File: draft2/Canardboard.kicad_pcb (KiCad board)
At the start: 4 copper layers, 96.5 x 62 mm, 112 parts, among them IC1 SIC437DED-T1-GE3, J1 RBUS, J2 USB_C_Receptacle_USB2.0, J3 Micro_SD_Card_Det, J4 Conn_01x02_Male, J5 Conn_01x03_Male, J6 Conn_01x03_Male, J7 Conn_01x03_Male, Q1 SI4143DY-T1-GE3, Q2 SI4143DY-T1-GE3, U1 ESP32-S3, U10 LTC4412xS6, U2 SN65HVD230, U3 LM66200DRLR, U5 MAX77827AEFD+T, U6 SC4215, U7 ICM-20608-G, U8 MMC5983MA, U9 LTC4412xS6, Y1 40MHz±10ppm

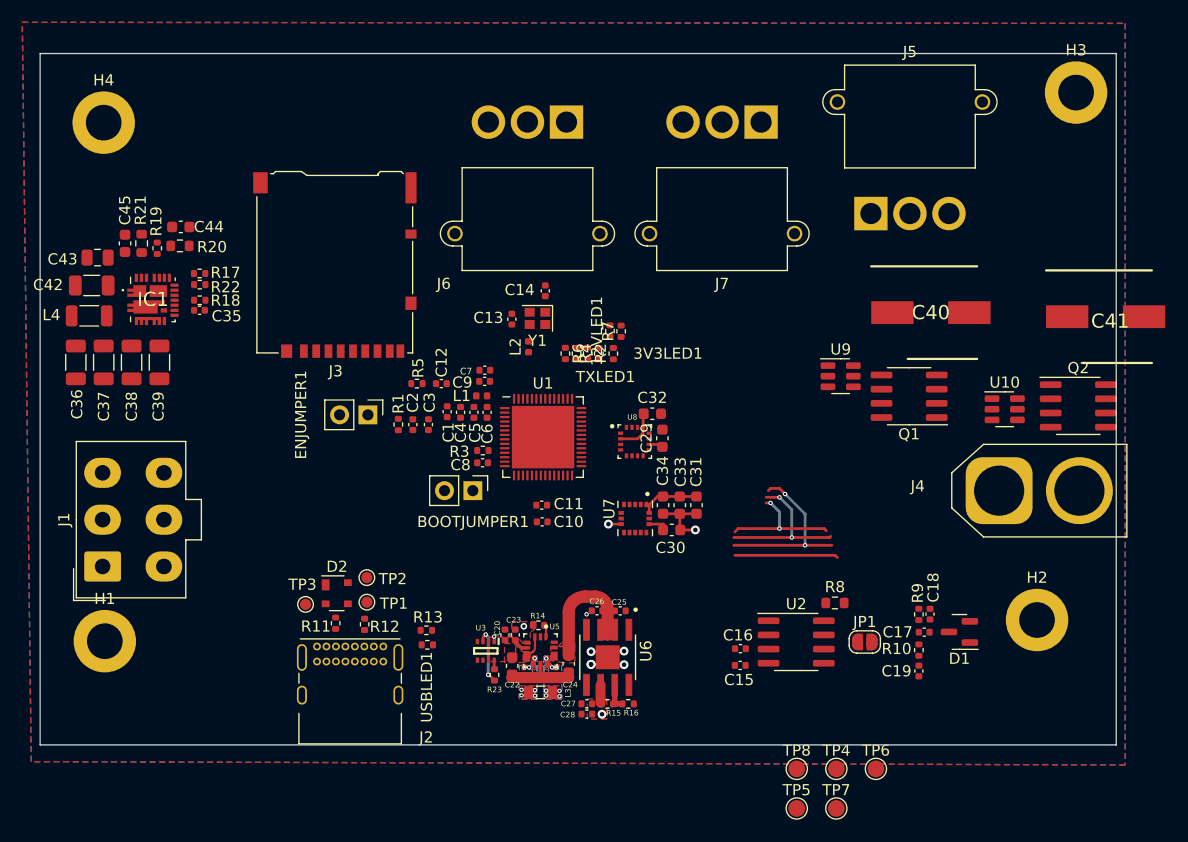
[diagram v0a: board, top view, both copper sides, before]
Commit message: made everything smaller
:)
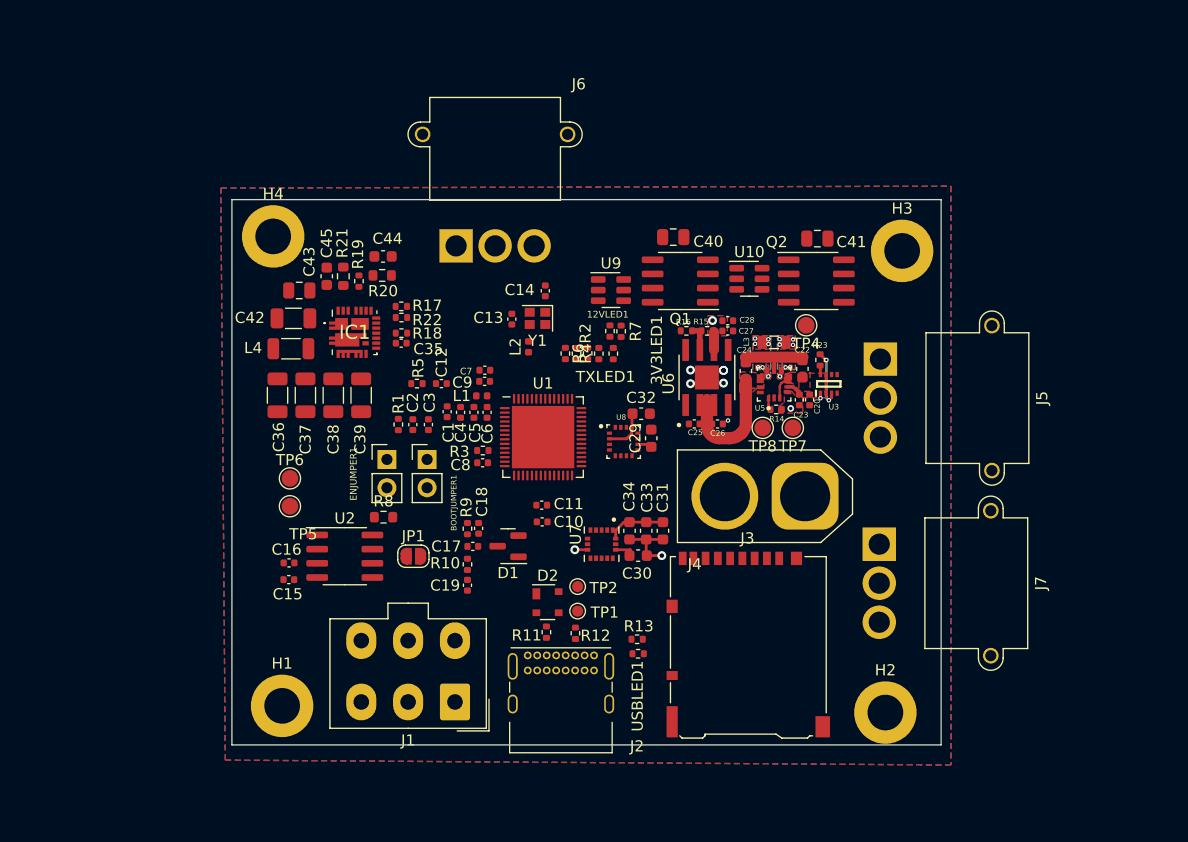
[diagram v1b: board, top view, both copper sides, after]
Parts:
- removed TP3: TestPoint, TestPoint:TestPoint_Pad_D1.0mm
- C40, C41: footprint iclr:CAPAE830X1050N -> Capacitor_SMD:C_0805_2012Metric
- moved TP6 58.7 mm to (102.2, 100.2)
- moved TP5 52.9 mm to (102.2, 102.7)
- moved J3 50.3 mm to (143.3, 115.1), turned to 0 degrees
- moved C15 41.2 mm to (102.1, 109.3)
- moved C17 41.2 mm to (118.6, 106.3)
- moved D1 41.2 mm to (121.8, 106.3)
- moved JP1 41.2 mm to (113.3, 107.2)
- moved C16 41.2 mm to (102.1, 107.8)
- moved C18 41.2 mm to (119.1, 104.7)
- moved C19 41.2 mm to (118.1, 109.8)
- moved R10 41.2 mm to (118.1, 107.9)
- moved R8 41.2 mm to (110.6, 103.7)
- moved R9 41.2 mm to (118.1, 104.7)
- moved U2 41.2 mm to (107.1, 107.2)
- moved R23 40.6 mm to (149.7, 89.6), turned to -90 degrees
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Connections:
- R23 pad 2: (no net) -> Net-(R23-Pad2)
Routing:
- net GND: track 64.4 -> 13.8 mm, vias 15 -> 10
- net VBUS: vias 3 -> 2
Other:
- board size 96.5 x 62 mm -> 63.6 x 48.9 mm
